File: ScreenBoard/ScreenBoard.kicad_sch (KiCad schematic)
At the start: 17 parts, among them J1 Conn_01x12_MountingPin, J2 LCD_FPC_0.7mm_welding, Q1 AO3415A, SW1 C318960, U1 XC6209

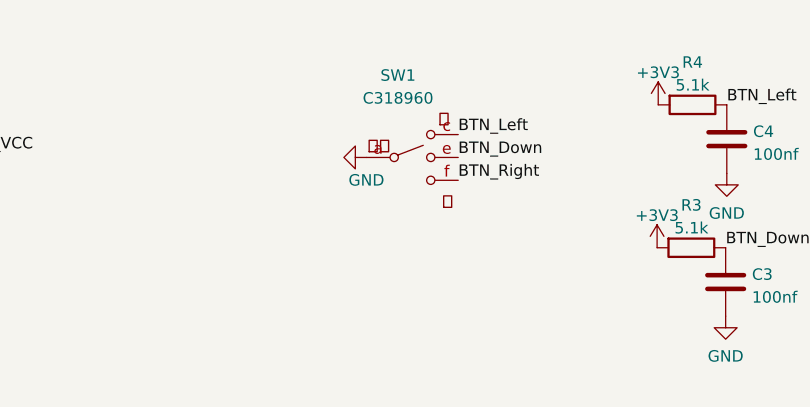
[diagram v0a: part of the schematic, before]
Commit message: 新款拨轮
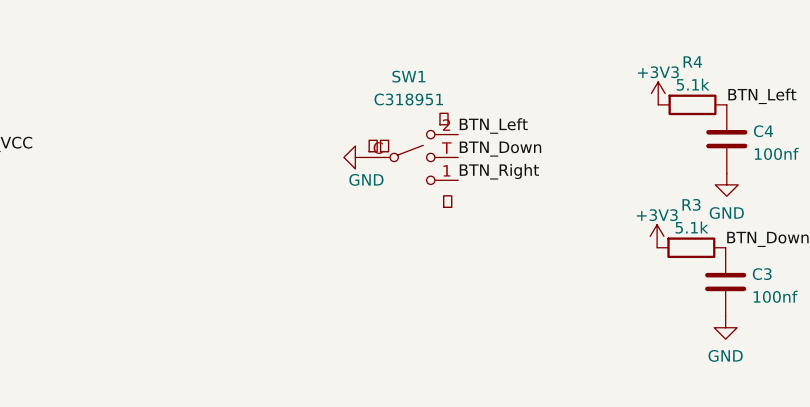
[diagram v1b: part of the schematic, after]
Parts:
- removed SW1: C318960, KisonNew:C318960, symbol KisonNew:C318960
- added SW1: C318951, KisonNew:C318951, symbol KisonNew:C318951
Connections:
- net BTN_Down: now also SW1.T
- net BTN_Left: now also SW1.2
- net BTN_Right: now also SW1.1
- net GND: now also SW1.C
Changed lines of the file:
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@@
     (pin "1")
+  )
+  (symbol (lib_id "KisonNew:C318951") (at 180.721 28.829 0) (unit 1)
+    (in_bom yes) (on_board yes) (fields_autoplaced)
+    (property "Reference" "SW1" (id 0) (at 180.3412 19.8983 0))
+    (property "Value" "C318951" (id 1) (at 180.3412 22.4352 0))
+    (property "Footprint" "KisonNew:C318951" (id 2) (at 164.846 24.384 0)
+      (effects (font (size 1.27 1.27)) hide)
+    )
+    (property "Datasheet" "~" (id 3) (at 164.846 24.384 0)
+      (effects (font (size 1.27 1.27)) hide)
+    )
+    (pin "1")
+    (pin "2")
+    (pin "C")
+    (pin "T")
   )
   (symbol (lib_id "power:GND") (at 104.775 57.785 180) (unit 1)
@@
     (pin "2")
   )
-  (symbol (lib_id "KisonNew:C318960") (at 180.721 28.829 0) (unit 1)
-    (in_bom yes) (on_board yes) (fields_autoplaced)
-    (property "Reference" "SW1" (id 0) (at 179.122 19.7205 0))
-    (property "Value" "C318960" (id 1) (at 179.122 22.2574 0))
-    (property "Footprint" "KisonNew:C318960" (id 2) (at 180.721 28.829 0)
-      (effects (font (size 1.27 1.27)) hide)
-    )
-    (property "Datasheet" "~" (id 3) (at 180.721 28.829 0)
-      (effects (font (size 1.27 1.27)) hide)
-    )
-    (pin "a")
-    (pin "c")
-    (pin "e")
-    (pin "f")
-  )
   (symbol (lib_id "power:GND") (at 235.077 30.48 0) (unit 1)
     (in_bom yes) (on_board yes) (fields_autoplaced)
@@
       (reference "R5") (unit 1) (value "5.1k") (footprint "Capacitor_SMD:C_0402_1005Metric")
     )
-    (path "/53f90dd5-3a0b-48eb-965c-6aaa765b9334"
-      (reference "SW1") (unit 1) (value "C318960") (footprint "KisonNew:C318960")
+    (path "/1dbe7728-308d-40ae-b824-b166c49fdb93"
+      (reference "SW1") (unit 1) (value "C318951") (footprint "KisonNew:C318951")
     )
     (path "/e25f0cb2-d101-4680-8039-e28dc3ef0e9b"

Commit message: Fix most 3D parts
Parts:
- J1: footprint Connector_FFC-FPC:Hirose_FH12-12S-0.5SH_1x12-1MP_P0.50mm_Horizontal -> KisonNew:Hirose_FH12-12S-0.5SH_1x12-1MP_P0.50mm_Horizontal
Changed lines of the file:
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@@
       (effects (font (size 1.27 1.27)) (justify left))
     )
-    (property "Footprint" "Connector_FFC-FPC:Hirose_FH12-12S-0.5SH_1x12-1MP_P0.50mm_Horizontal" (id 2) (at 28.575 34.925 0)
+    (property "Footprint" "KisonNew:Hirose_FH12-12S-0.5SH_1x12-1MP_P0.50mm_Horizontal" (id 2) (at 28.575 34.925 0)
       (effects (font (size 1.27 1.27)) hide)
     )
@@
     )
     (path "/483f7aee-8377-41a9-be2e-d078c58ff352"
-      (reference "J1") (unit 1) (value "Conn_01x12_MountingPin") (footprint "Connector_FFC-FPC:Hirose_FH12-12S-0.5SH_1x12-1MP_P0.50mm_Horizontal")
+      (reference "J1") (unit 1) (value "Conn_01x12_MountingPin") (footprint "KisonNew:Hirose_FH12-12S-0.5SH_1x12-1MP_P0.50mm_Horizontal")
     )
     (path "/97181880-94fa-42d4-b759-0e5452e90cce"
